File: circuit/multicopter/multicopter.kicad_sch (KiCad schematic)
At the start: 21 parts, among them J1 Conn_01x02_Male, SW1 SW_Push, U1 ESP32-DEVKITC-32E, U2 MT3608, U4 BNO055

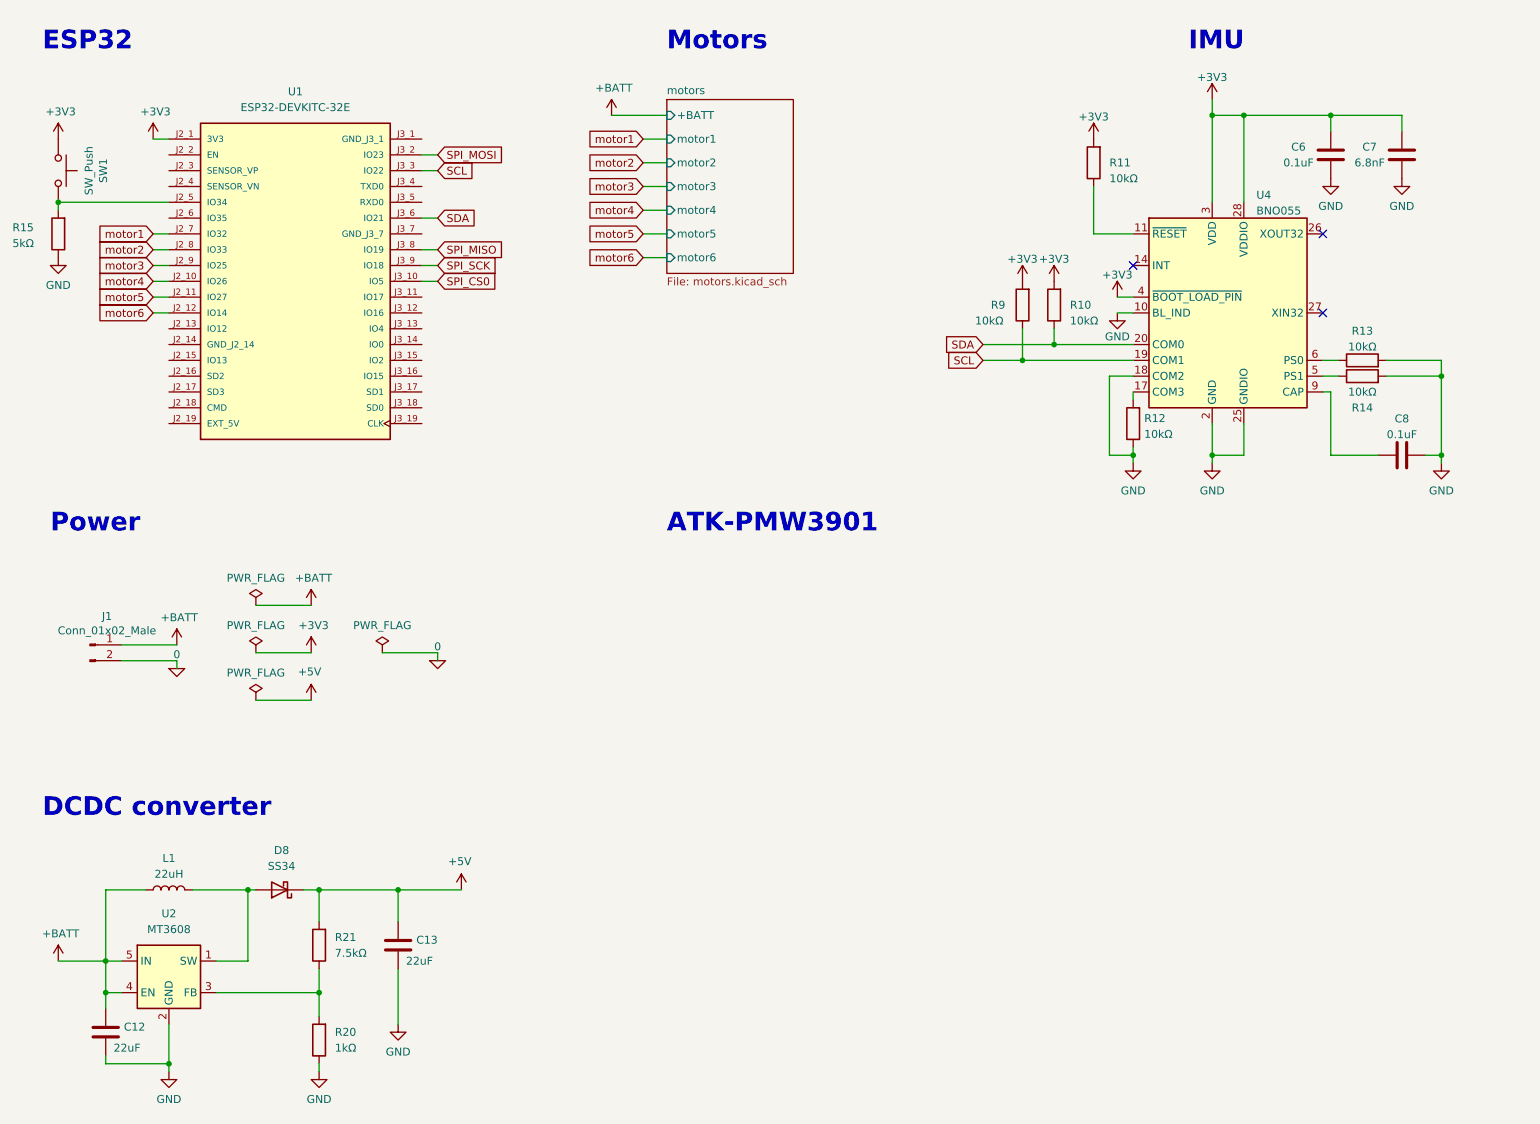
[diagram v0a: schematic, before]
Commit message: completed schematic.
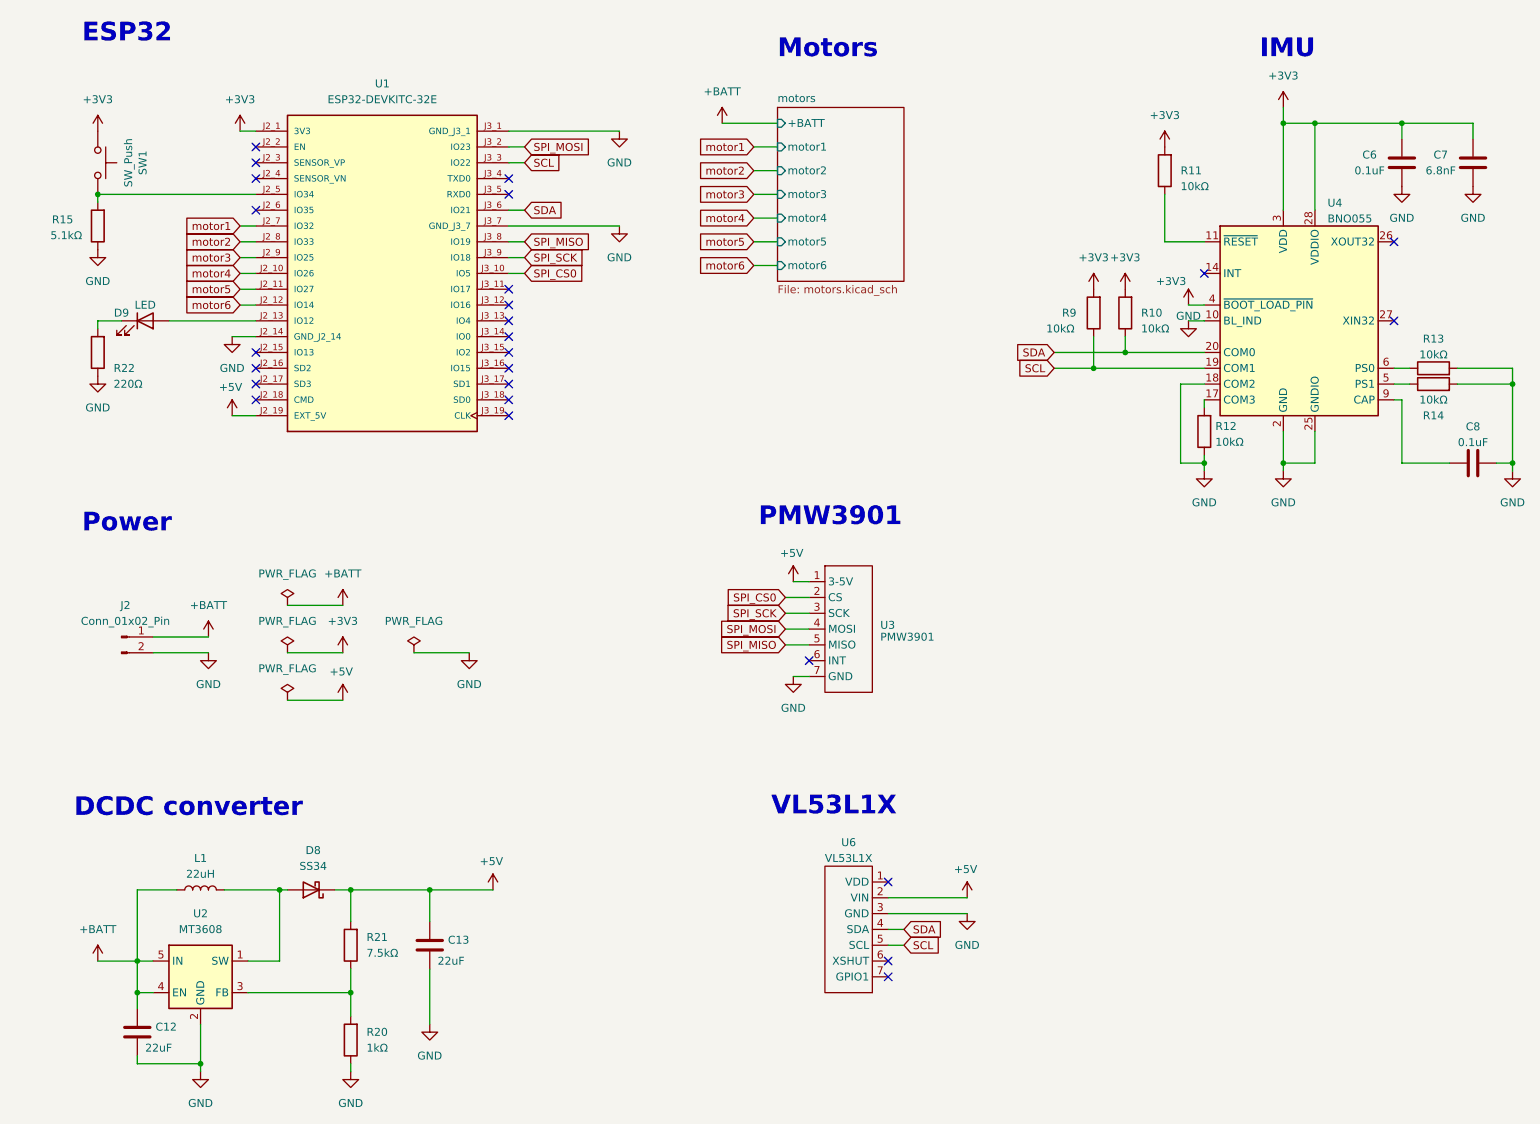
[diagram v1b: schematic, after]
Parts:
- removed J1: Conn_01x02_Male, Connector_PinHeader_2.54mm:PinHeader_1x02_P2.54mm_Vertical, symbol flightcontroller-rescue:Conn_01x02_Male-Connector
- added D9: LED, Diode_SMD:D_0603_1608Metric, symbol Device:LED
- added J2: Conn_01x02_Pin, symbol Connector:Conn_01x02_Pin
- added R22: 220Ω, Resistor_SMD:R_0603_1608Metric, symbol Device:R
- added U3: PMW3901, symbol drone2:PIM453_PMW3901
- added U6: VL53L1X, symbol drone2:POLOLU-3415_VL53L1X
- R15: value 5kΩ -> 5.1kΩ
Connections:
- net +5V: now also U1.J2_19 (EXT_5V), U3.1 (3-5V), U6.2 (VIN)
- net +BATT: now also J2.1 (Pin_1)
- net GND: now also U1.J2_14 (GND_J2_14), U1.J3_1 (GND_J3_1), U1.J3_7 (GND_J3_7), J2.2 (Pin_2), R22.1, U3.7 (GND), U6.3 (GND); no longer U4.15 (GNDIO), U4.16 (GNDIO)
- net SCL: now also U6.5 (SCL)
- net SDA: now also U6.4 (SDA)
- net SPI_CS0: now also U3.2 (CS)
- net SPI_MISO: now also U3.5 (MISO)
- net SPI_MOSI: now also U3.4 (MOSI)
- net SPI_SCK: now also U3.3 (SCK)
- net at U1.J2_13 (IO12): now also D9.2 (A)
- new net: D9.1 (K), R22.2
- no-connect marks 3 -> 26
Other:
- note added: "PMW3901"
- note added: "VL53L1X"
- note removed: "ATK-PMW3901"
- moved on the sheet: C12, C13, C6, C7, C8, D8, L1, R10, R11, R12, R13, R14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

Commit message: added circuits.
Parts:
- C12, C13: MANUFACTURER (none) -> KYOCERA AVX; Mounting Type (none) -> SMD; Production Number (none) -> 0603ZD226MAT2A; Purchase link (none) -> https://www.mouser.jp/ProductDetail/KYOCERA-AVX/0603ZD226MA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; Unit Price (none) -> 85.8
- C6, C8: MANUFACTURER (none) -> KYOCERA AVX; Mounting Type (none) -> SMD; Production Number (none) -> KAM15AR71C104KM; Purchase link (none) -> https://www.mouser.jp/ProductDetail/KYOCERA-AVX/KAM15AR71C1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; Unit Price (none) -> 56.1
- C7: MANUFACTURER (none) -> Vishay / Vitramon; Mounting Type (none) -> SMD; Production Number (none) -> VJ0603Y682KXBAC31X; Purchase link (none) -> https://www.mouser.jp/ProductDetail/Vishay-Vitramon/VJ0603Y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; Unit Price (none) -> 41.3
- D8: footprint Diode_SMD:D_SMC -> Diode_SMD:D_SOD-123F; MANUFACTURER (none) -> onsemi / Fairchild; Mounting Type (none) -> SMD; Production Number (none) -> SS34FA; Purchase link (none) -> https://www.mouser.jp/ProductDetail/onsemi-Fairchild/SS34FA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; Unit Price (none) -> 62.7; Vendor (none) -> https://www.mouser.jp/ProductDetail/onsemi-Fairchild/SS34?q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
- D9: MANUFACTURER (none) -> Bivar; Mounting Type (none) -> SMD; Production Number (none) -> SM0603UBWC; Purchase link (none) -> https://www.mouser.jp/ProductDetail/Bivar/SM0603UBWC?qs=hWD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; Unit Price (none) -> 242.6
- J2: footprint (none) -> Connector_PinHeader_2.54mm:PinHeader_1x02_P2.54mm_Vertical; Mounting Type (none) -> THT
- L1: MANUFACTURER (none) -> Vishay / Dale; Mounting Type (none) -> SMD; Production Number (none) -> IHLP2020BZER220M5A; Purchase link (none) -> https://www.mouser.jp/ProductDetail/Vishay-Dale/IHLP2020BZE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; Unit Price (none) -> 207.9
- R10, R11, R12, R13, R14, R9: MANUFACTURER (none) -> Vishay / Beyschlag; Mounting Type (none) -> SMD; Production Number (none) -> MCT06030D1002BP500; Purchase link (none) -> https://www.mouser.jp/ProductDetail/Vishay-Beyschlag/MCT060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; Unit Price (none) -> 23.1
- R15: MANUFACTURER (none) -> Vishay / Dale; Mounting Type (none) -> SMD; Production Number (none) -> CRCW06035K10FKEC; Purchase link (none) -> https://www.mouser.jp/ProductDetail/Vishay-Dale/CRCW06035K1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; Unit Price (none) -> 19.8
- R20: MANUFACTURER (none) -> TDK; Mounting Type (none) -> SMD; Production Number (none) -> MMZ1608S102ATA00; Purchase link (none) -> https://www.mouser.jp/ProductDetail/TDK/MMZ1608S102ATA00?qs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; Unit Price (none) -> 16.5
- R21: MANUFACTURER (none) -> Susumu; Mounting Type (none) -> SMD; Production Number (none) -> RG1608P-752-B-T5; Purchase link (none) -> https://www.mouser.jp/ProductDetail/Susumu/RG1608P-752-B-T5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; Unit Price (none) -> 34.7
- R22: MANUFACTURER (none) -> Pulse Electronics; Mounting Type (none) -> SMD; Production Number (none) -> GBK160808T-221Y-N; Purchase link (none) -> https://www.mouser.jp/ProductDetail/Pulse-Electronics/GBK16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; Unit Price (none) -> 16.5
- SW1: footprint Button_Switch_THT:SW_PUSH_6mm_H5mm -> Button_Switch_SMD:SW_Push_1P1T_NO_CK_KMR2; MANUFACTURER (none) -> C&K; Mounting Type (none) -> SMD; Production Number (none) -> KMR231NGLFS; Purchase link (none) -> https://www.mouser.jp/ProductDetail/CK/KMR231NGLFS?qs=sb%25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; Unit Price (none) -> 137
- U1: MANUFACTURER Espressif Systems -> CXH; Mounting Type (none) -> THT; Purchase link (none) -> https://www.alibaba.com/product-detail/2-54mm-Pitch-1x19-pi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; Unit Price (none) -> 74.66
- U2: MANUFACTURER (none) -> CYLDCHIP; Mounting Type (none) -> SMD; Production Number (none) -> MT3608; Purchase link (none) -> https://ja.aliexpress.com/item/1005005498022711.html?src=go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; Unit Price (none) -> 53
- U3, U6: footprint (none) -> Connector_JST:JST_PH_B7B-PH-K_1x07_P2.00mm_Vertical; MANUFACTURER (none) -> JST Sales America Inc.; Mounting Type (none) -> THT; Production Number (none) -> B7B-PH-K-S; Purchase link (none) -> https://www.digikey.jp/ja/products/detail/jst-sales-america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; Unit Price (none) -> 50.77
- U4: MANUFACTURER (none) -> Bosch Sensortec; Mounting Type (none) -> SMD; Production Number (none) -> BNO055; Purchase link (none) -> https://www.mouser.jp/ProductDetail/Bosch-Sensortec/BNO055?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; Unit Price (none) -> 2,036.1
